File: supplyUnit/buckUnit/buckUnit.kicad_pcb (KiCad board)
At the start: 2 copper layers, 72.7 x 33.9 mm, 25 parts, among them J1 12V, J10 SPARE, J11 Conn_01x05, J2 GND, J3 VBAT, J4 Motor, J5 Drib A, J6 Drib B, J7 L1, J8 SPARE, J9 L1, U1 OKL-T6-W12P-C, U2 OKL-T6-W12P-C

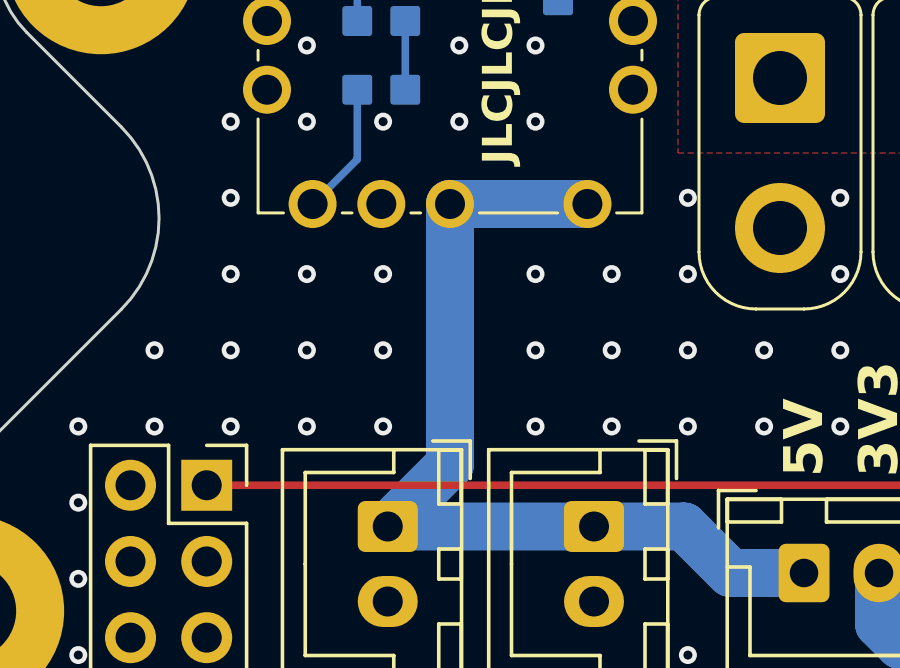
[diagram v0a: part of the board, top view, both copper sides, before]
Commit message: Fab
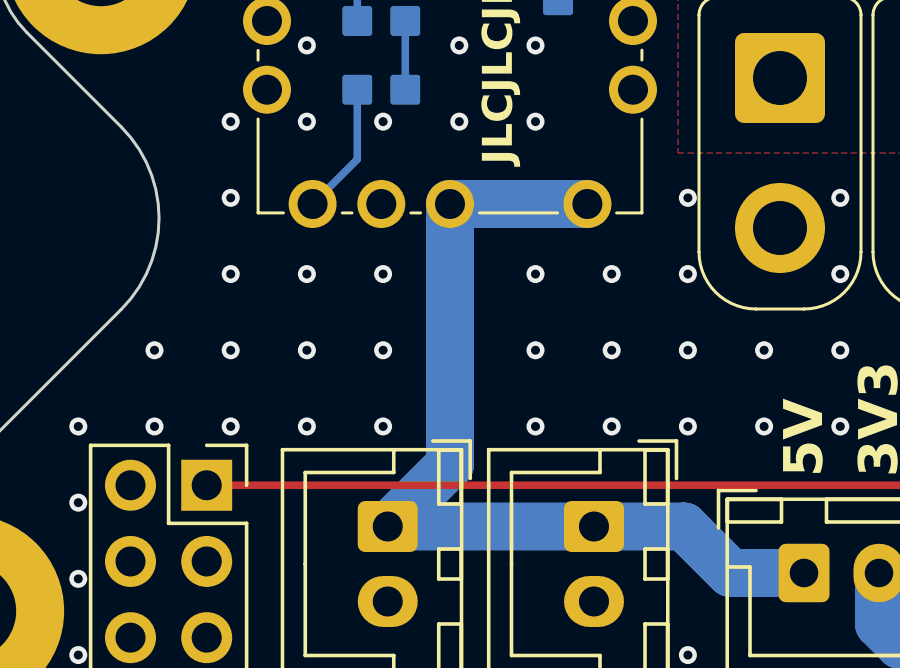
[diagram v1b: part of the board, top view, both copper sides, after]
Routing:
- net +3V3: track 36.5 -> 30.7 mm
